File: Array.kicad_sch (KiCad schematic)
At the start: 3 parts

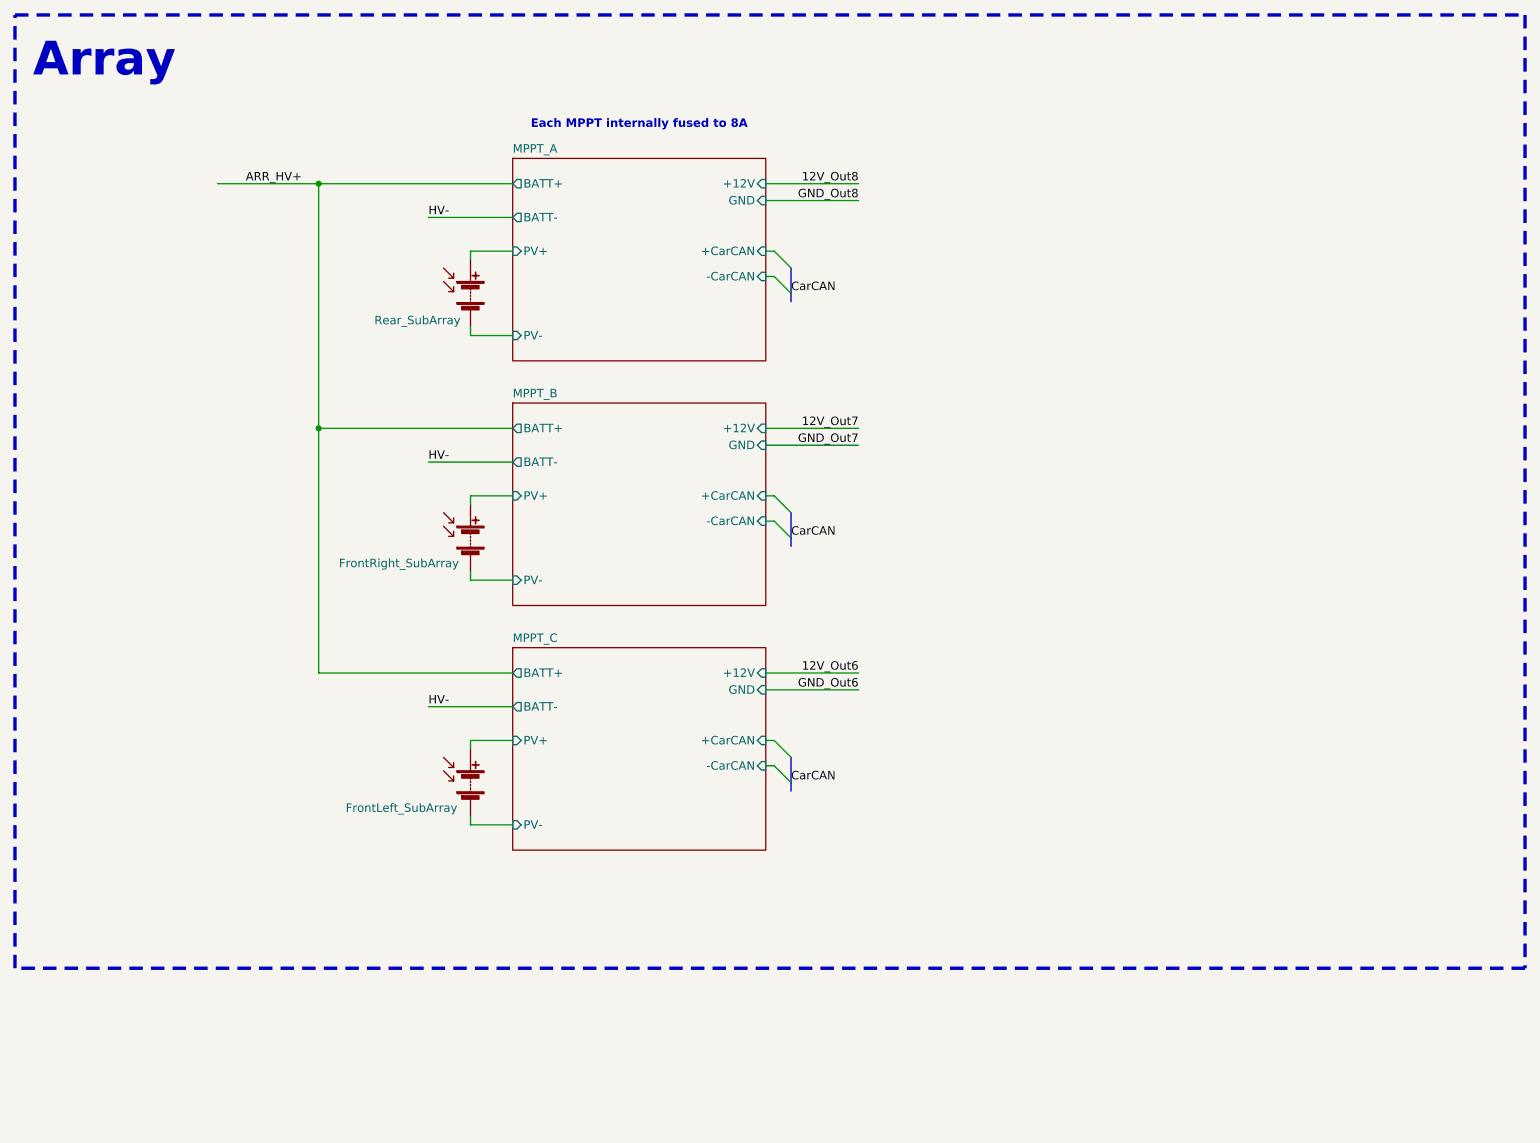
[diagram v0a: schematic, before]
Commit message: array stuff
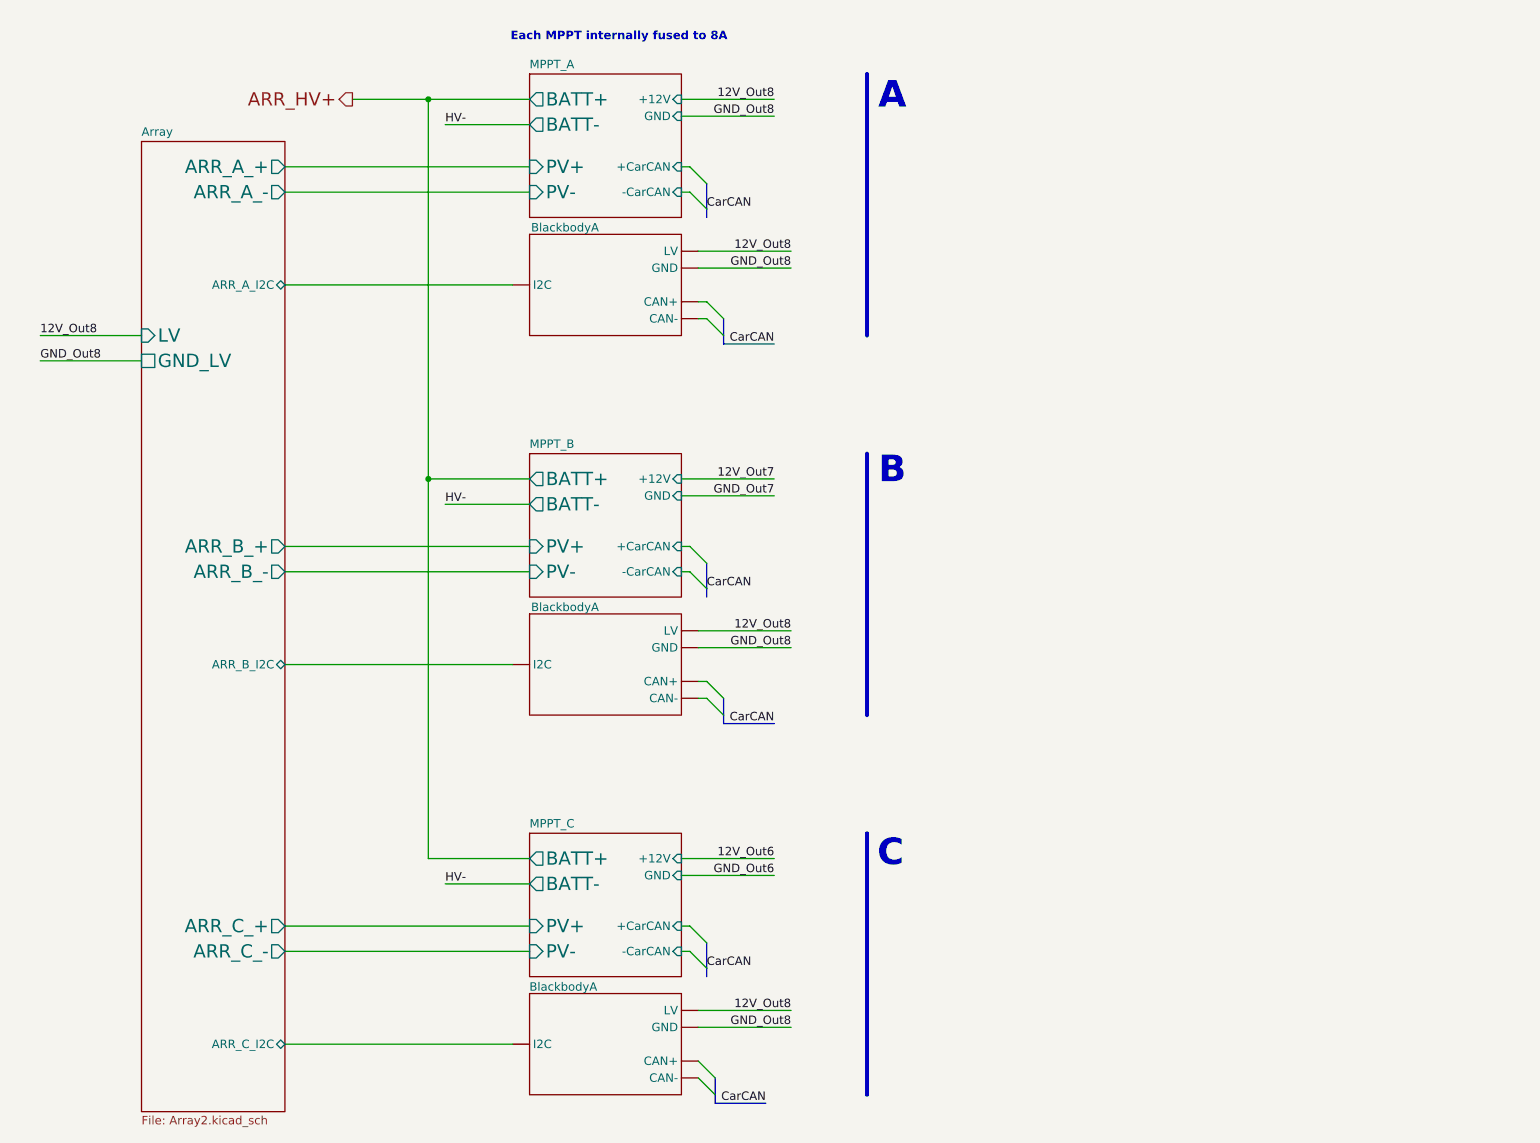
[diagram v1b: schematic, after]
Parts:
- removed SC3: FrontLeft_SubArray, symbol Device:Solar_Cells
- removed SC4: FrontRight_SubArray, symbol Device:Solar_Cells
- removed SC5: Rear_SubArray, symbol Device:Solar_Cells
- added U13, U14, U7: BlackbodyA, symbol lib:BlackbodyA
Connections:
- net 12V_Out8: now also U13. (CAN-), U14. (CAN-), U7. (CAN-)
- net GND_Out8: now also U13. (CAN-), U14. (CAN-), U7. (CAN-)
- new net Array/ARR_A_I2C: U7. (CAN-)
- new net Array/ARR_B_I2C: U13. (CAN-)
- new net Array/ARR_C_I2C: U14. (CAN-)
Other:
- added sheet Array (Array2.kicad_sch)
- note added: "A"
- note added: "B"
- note added: "C"
- note removed: "Array"
